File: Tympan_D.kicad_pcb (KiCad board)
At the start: 4 copper layers, 38 x 74 mm, 116 parts, among them IC1 MK66FX1M0VMD18, IC2 MKL02Z32VFG4, IC3 BC127, J1 SJ-3523-SMT-TR, J2 SJ-3524-SMT-TR-PI, J3 alt Power Pads, P1 USB_OTG, P10 CONN_01X01, P2 CONN_01X06, P3 CONN_01X06, P4 CONN_01X06, P5 CONN_01X06, P6 CONN_01X03, P7 CONN_01X01, P8 CONN_01X01, P9 CONN_01X01, SW1 CL-SB-22A, SW2 TACT_SWITCH, U1 AP2210K-3.3TRG1, U2 TLV320AIC3206IRSBT, U3 74LVC1G66, U4 LP5907MFX-1.8, U5 MCP73831, Y1 32.768kHz, Y2 16MHz

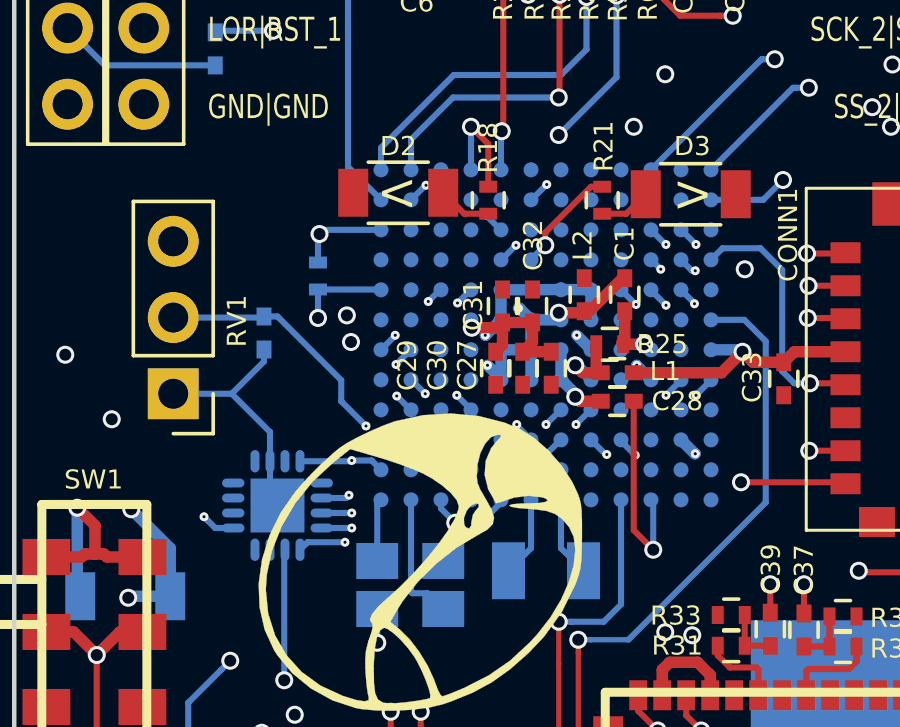
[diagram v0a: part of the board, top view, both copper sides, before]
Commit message: DMF changes for HiQ electronics bangalore
DMF changes for HiQ electronics bangalore
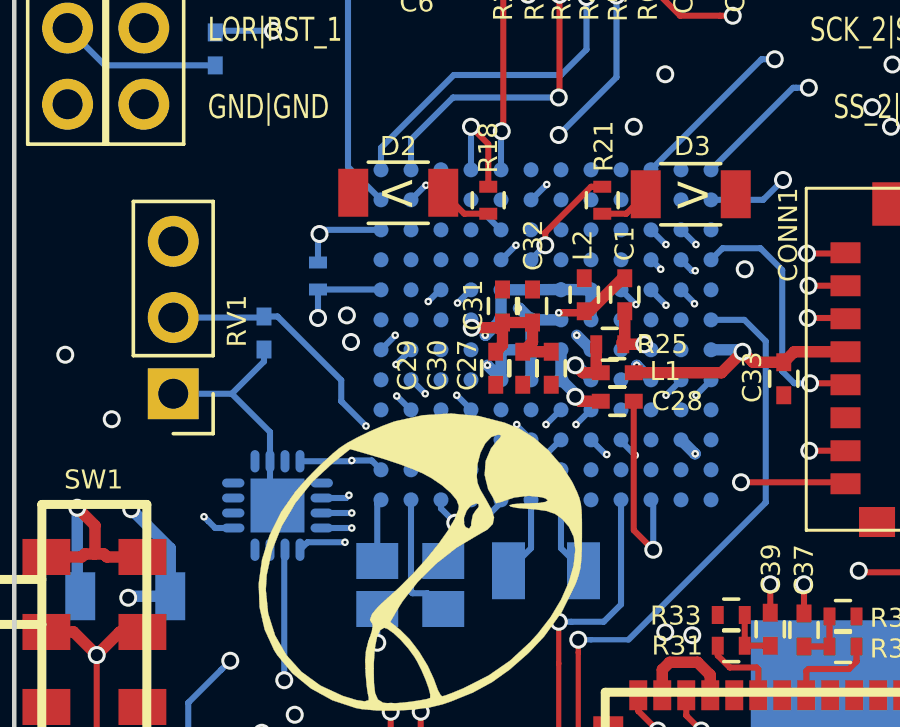
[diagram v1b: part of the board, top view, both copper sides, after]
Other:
- rule via_min_drill: 0.3 -> 0.1
- rule via_min_size: 0.4 -> 0.2
